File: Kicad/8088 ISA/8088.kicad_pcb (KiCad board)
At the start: 2 copper layers, 132 x 73.9 mm, 28 parts, among them J1 Conn_02x08_Counter_Clockwise, J9 Bus_ISA_8bit, U1 8284, U2 74LS573, U3 74LS573, U4 74LS245, U5 8088, U6 8259, U7 8253, U8 74LS257, Y1 Crystal

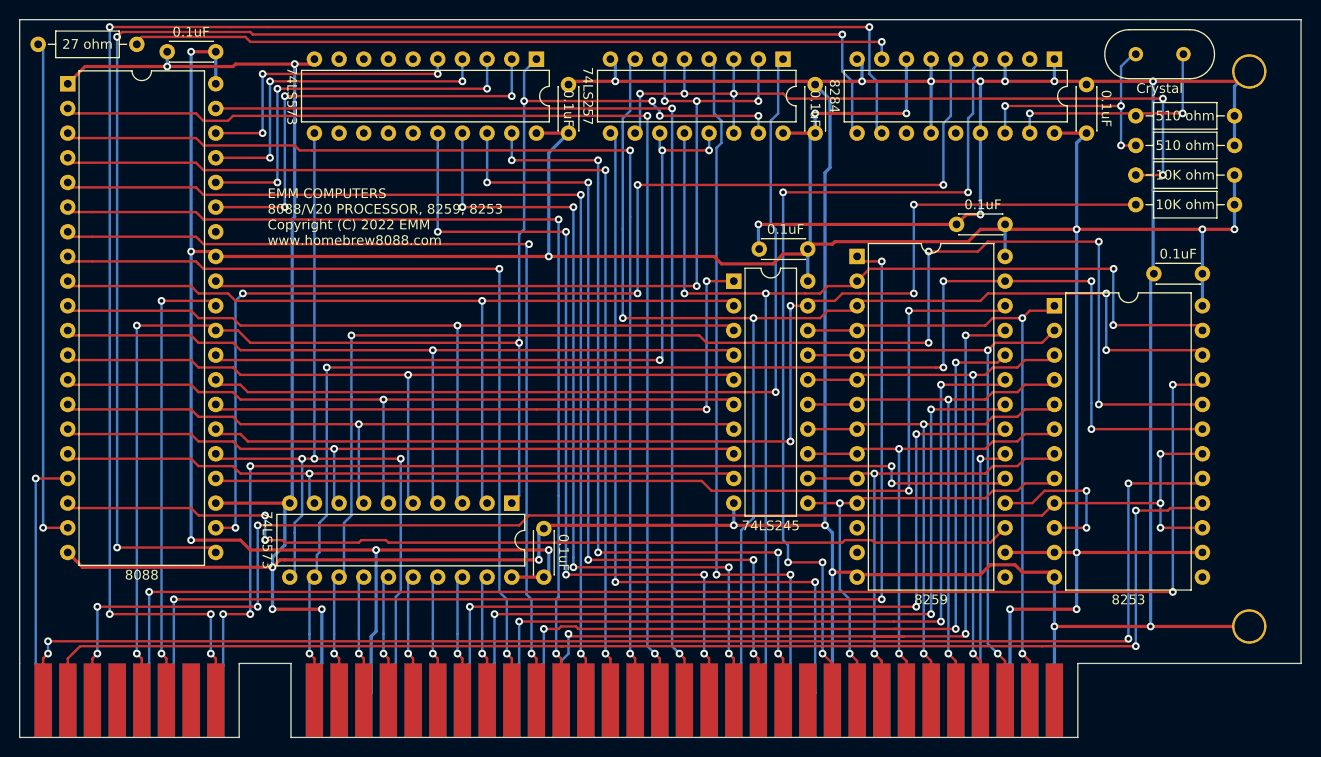
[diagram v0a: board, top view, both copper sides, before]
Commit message: update 8088 card
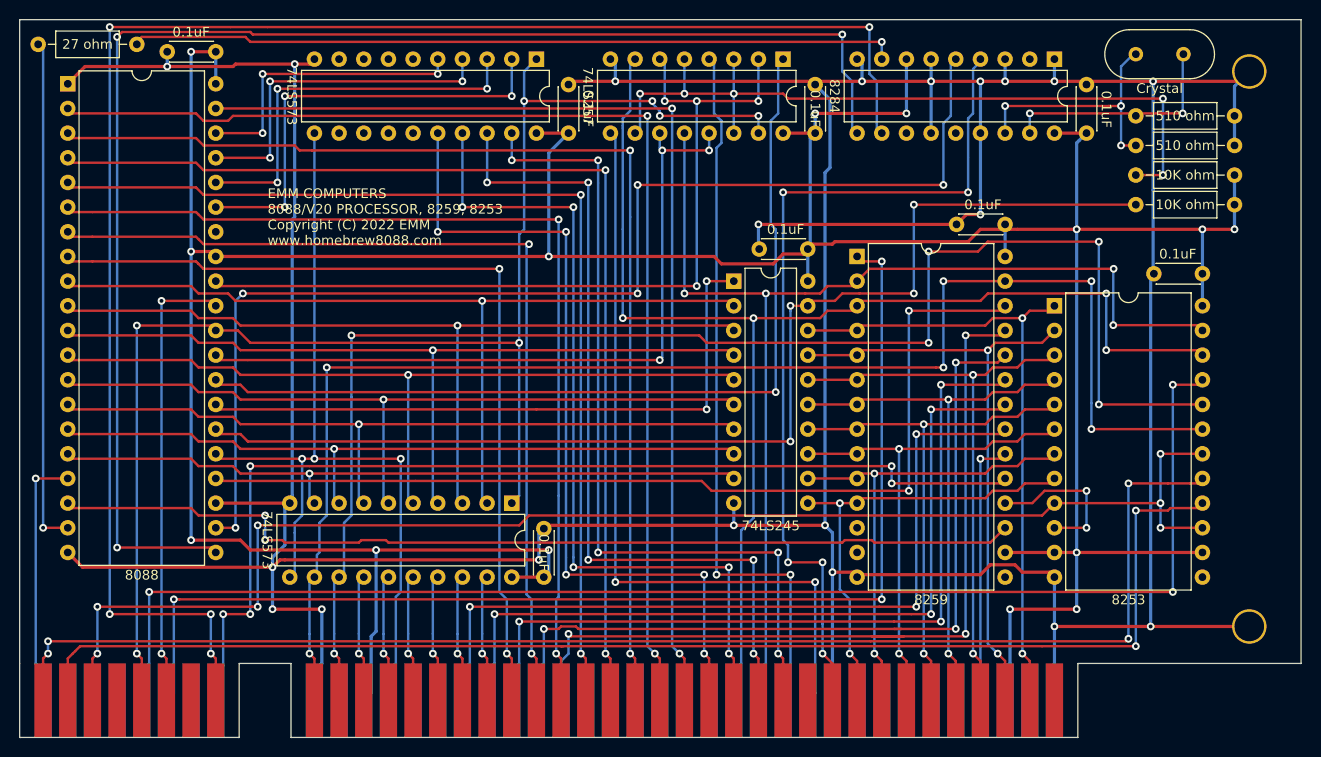
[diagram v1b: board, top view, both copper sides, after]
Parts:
- moved C2 45.8 mm to (111.5, 66.3)
- moved C3 45.8 mm to (109.0, 112.1)
- moved C8 39.9 mm to (171.8, 85.8), turned to 0 degrees
- moved C5 27.9 mm to (136.9, 66.3)
- moved C6 20.7 mm to (164.8, 66.3), turned to 270 degrees
- renumbered R2 to R1, R4 to R2, R5 to R4, R1 to R5, U5 to U1, U3 to U2, U2 to U3, U8 to U5, U1 to U6, U6 to U7, U7 to U8
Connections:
- net /PCLK88 renamed Net-(J1-Pad7)
